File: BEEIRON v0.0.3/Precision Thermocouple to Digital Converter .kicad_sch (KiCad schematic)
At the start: 17 parts, among them U6 MAX31856

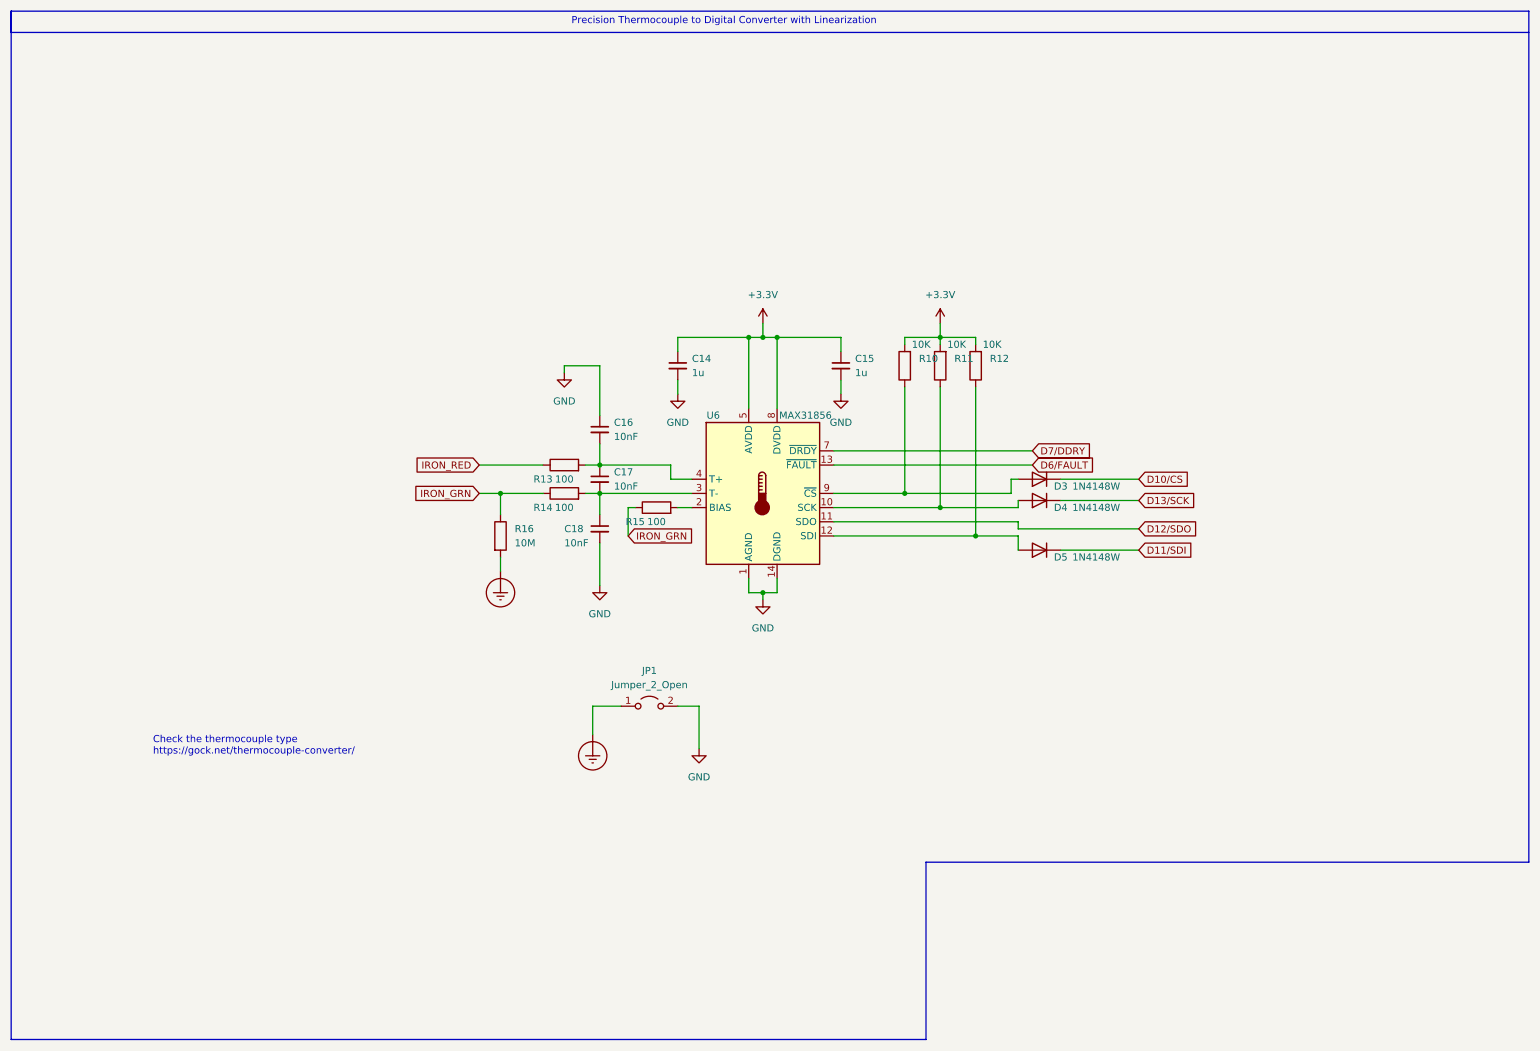
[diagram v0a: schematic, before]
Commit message: added bakup file
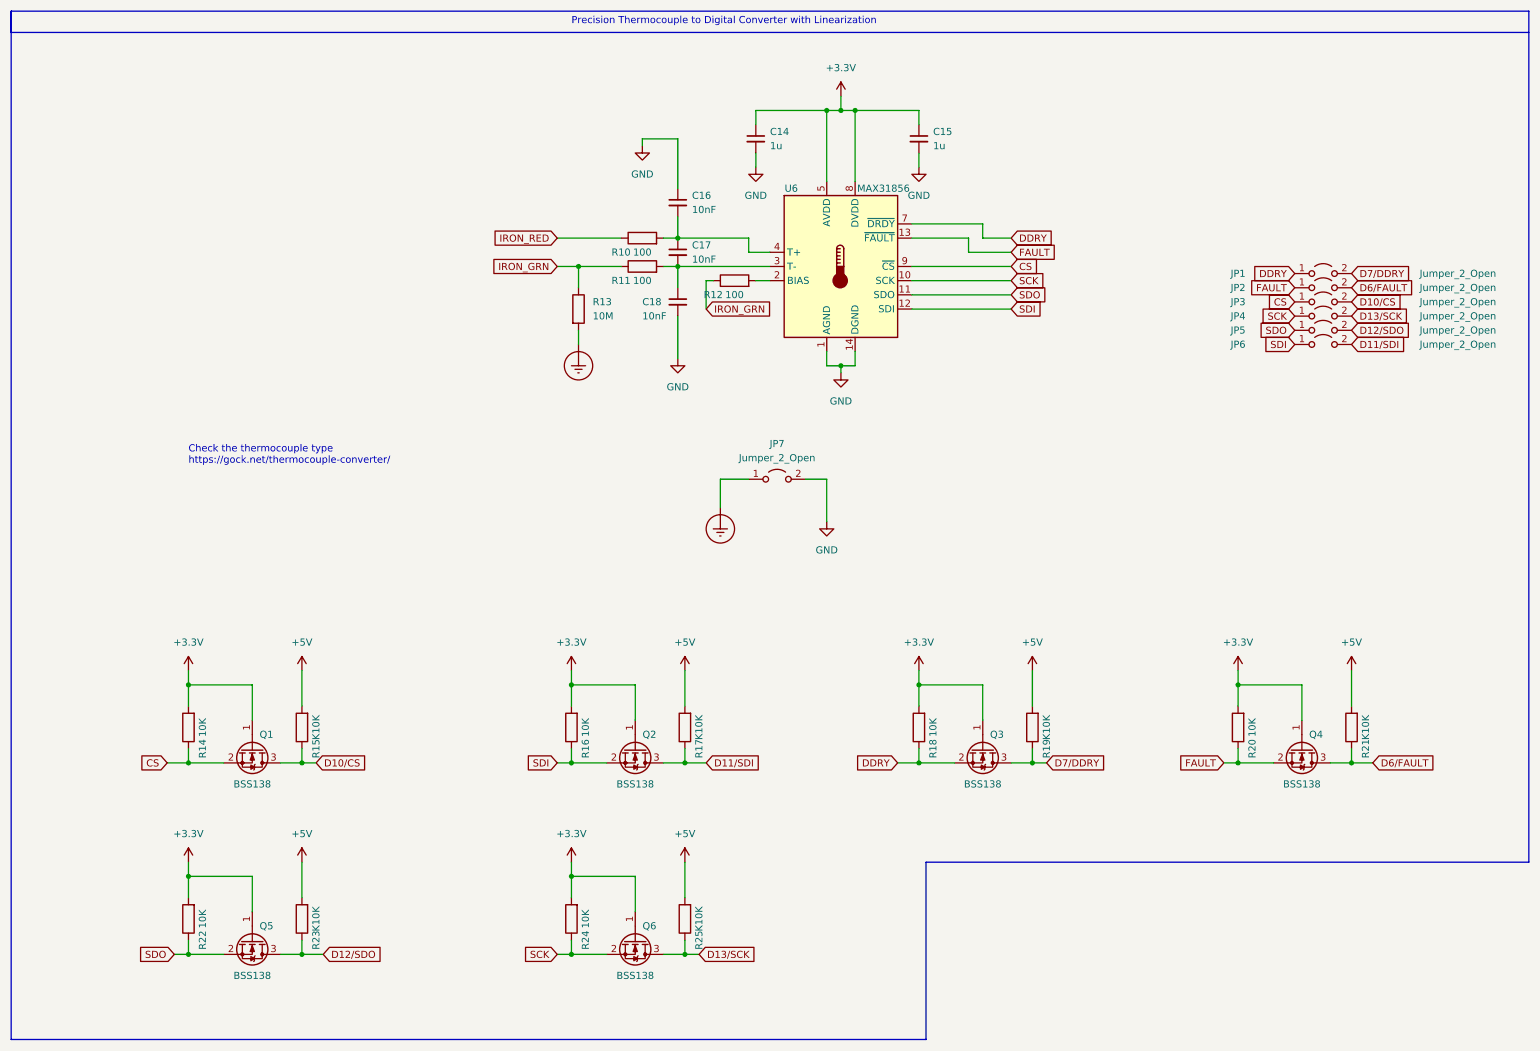
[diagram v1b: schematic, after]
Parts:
- removed D3, D4, D5: 1N4148W, Diode_SMD:D_SOD-123, symbol Diode:1N4148W
- removed R10, R11, R12: 10K, Resistor_SMD:R_0805_2012Metric, symbol Device:R
- added JP1, JP2, JP3, JP4, JP5, JP6: Jumper_2_Open, Jumper:SolderJumper-2_P1.3mm_Open_TrianglePad1.0x1.5mm, symbol Jumper:Jumper_2_Open
- added Q1, Q2, Q3, Q4, Q5, Q6: BSS138, Package_TO_SOT_SMD:SOT-23, symbol Transistor_FET:BSS138
- added R14, R16, R18, R20, R22, R24: 10K, Resistor_SMD:R_0805_2012Metric, symbol Device:R
- added R15, R17, R19, R21, R23, R25: K10K, Resistor_SMD:R_0805_2012Metric, symbol Device:R
- renumbered JP1 to JP7, R13 to R10, R14 to R11, R15 to R12, R16 to R13
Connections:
- net +3V3: now also Q1.1 (G), Q2.1 (G), Q3.1 (G), Q4.1 (G), Q5.1 (G), Q6.1 (G), R14.2, R16.2, R18.2, R20.2, R22.2, R24.2
- net D10/CS: now also JP3.2 (B), Q1.3 (D), R15.1
- net D11/SDI: now also JP6.2 (B), Q2.3 (D), R17.1
- net D12/SDO: now also JP5.2 (B), Q5.3 (D), R23.1; no longer U6.11 (SDO)
- net D13/SCK: now also JP4.2 (B), Q6.3 (D), R25.1
- net D6/FAULT: now also JP2.2 (B), Q4.3 (D), R21.1; no longer U6.13 (~{FAULT})
- net D7/DDRY: now also JP1.2 (B), Q3.3 (D), R19.1; no longer U6.7 (~{DRDY})
- net CS: now reaches U6.9 (~{CS})
- net CS: now also JP3.1 (A), Q1.2 (S), R14.1
- net SCK: now reaches U6.10 (SCK)
- net SCK: now also JP4.1 (A), Q6.2 (S), R24.1
- net SDI: now reaches U6.12 (SDI)
- net SDI: now also JP6.1 (A), Q2.2 (S), R16.1
- new net +5V: R15.2, R17.2, R19.2, R21.2, R23.2, R25.2
- new net DDRY: JP1.1 (A), Q3.2 (S), R18.1, U6.7 (~{DRDY})
- new net FAULT: JP2.1 (A), Q4.2 (S), R20.1, U6.13 (~{FAULT})
- new net SDO: JP5.1 (A), Q5.2 (S), R22.1, U6.11 (SDO)
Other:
- moved on the sheet: C14, C15, C16, C17, C18, JP7, R10, R11, R12, R13, U6
